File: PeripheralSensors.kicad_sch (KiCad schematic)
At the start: 17 parts, among them J19 TOF_Connectors, J21 IMU_Conn, U2 SAM-M8Q, U4 SP3011-06UTG, U5 SP3011-06UTG, U6 SP3011-06UTG

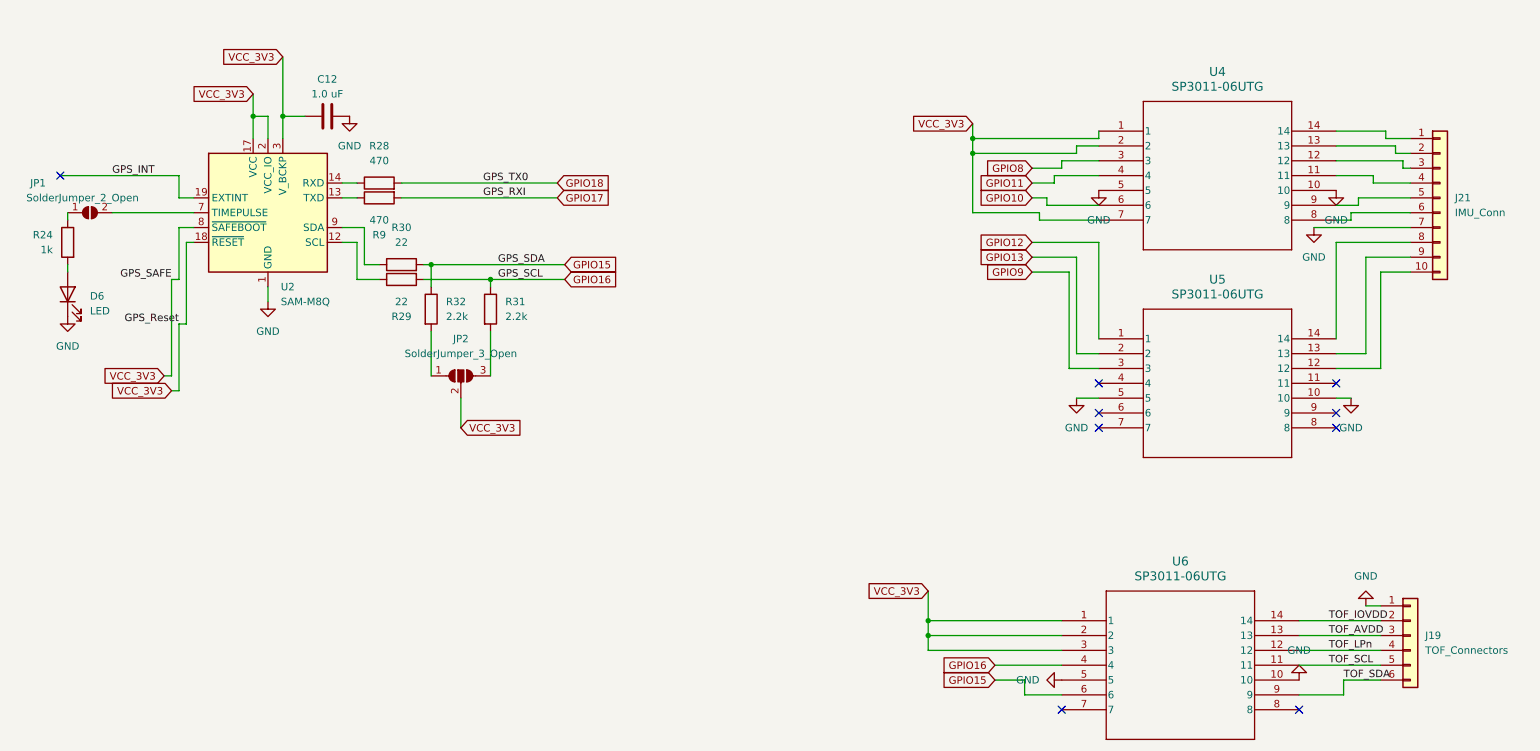
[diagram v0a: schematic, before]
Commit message: pcb draft 2 from billy
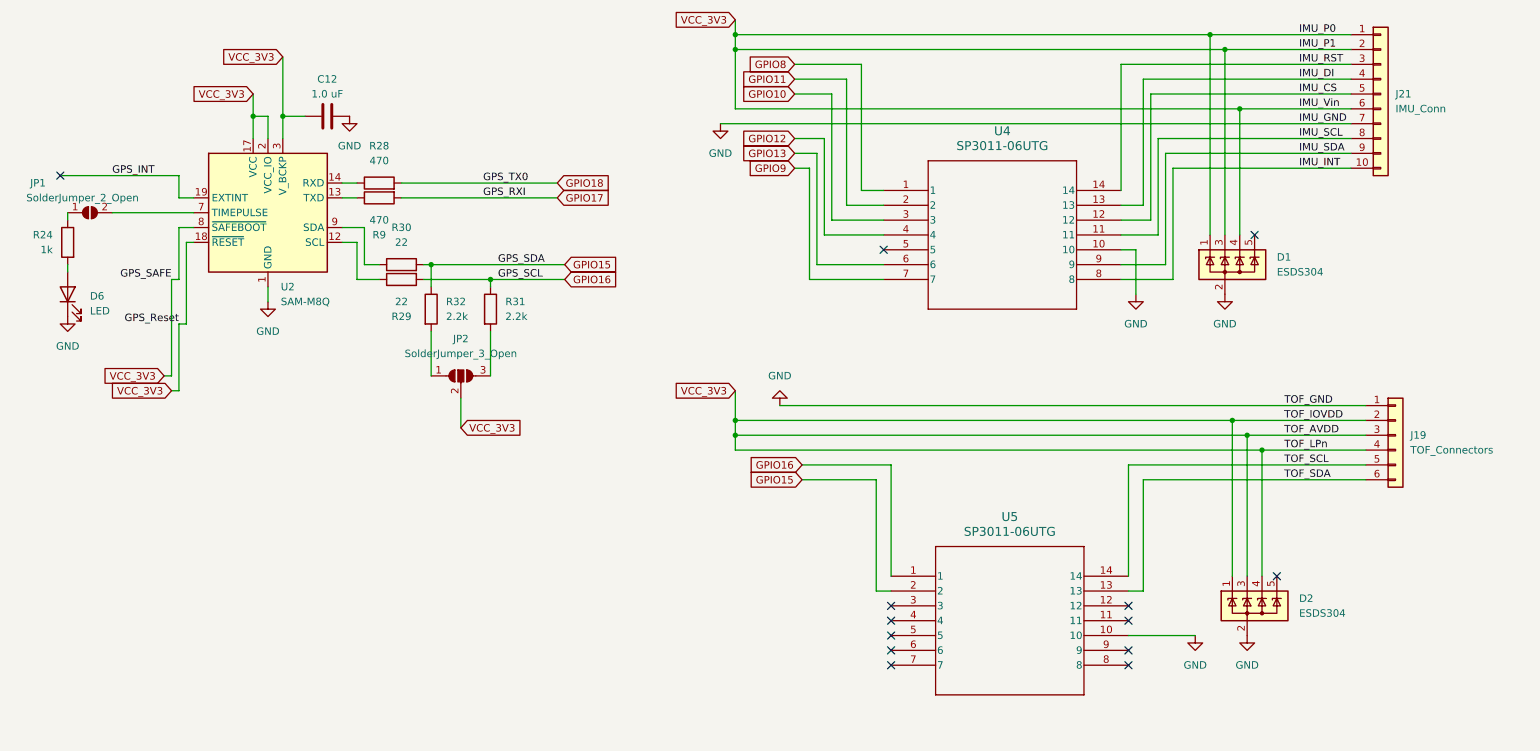
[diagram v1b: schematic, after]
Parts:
- removed U4, U5, U6: SP3011-06UTG, LocalComponents:SON14_SP3011-06UTG_LTF, symbol LocalComps:SP3011-06UTG
- added D1, D2: ESDS304, Package_TO_SOT_SMD:SOT-23-5, symbol Power_Protection:ESDS304
- added U4, U5: SP3011-06UTG, LocalComponents:SON14_SP3011-06UTG_LTF, symbol Custom_Components:SP3011-06UTG
- D6: footprint LocalComponents:LED_LTST-C171_LTO -> LED_SMD:LED_0201_0603Metric
- R24: footprint LocalComponents:RESC1508X55N -> Resistor_SMD:R_0805_2012Metric_Pad1.20x1.40mm_HandSolder
- R28, R9: footprint LocalComponents:RESC6332X65N -> Resistor_SMD:R_0805_2012Metric_Pad1.20x1.40mm_HandSolder
- R29, R30: footprint LocalComponents:R0402 -> Resistor_SMD:R_0805_2012Metric_Pad1.20x1.40mm_HandSolder
- R31, R32: footprint LocalComponents:RESC1005X35N -> Resistor_SMD:R_0805_2012Metric_Pad1.20x1.40mm_HandSolder
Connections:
- net TOF_AVDD is gone; now on net VCC_3V3: J19.3 (Pin_3)
- net TOF_IOVDD is gone; now on net VCC_3V3: J19.2 (Pin_2)
- net TOF_LPn is gone; now on net VCC_3V3: J19.4 (Pin_4)
- net GND: now also D1.2 (A), D2.2 (A), U4.10, U5.10
- net GPIO10: now also U4.3
- net GPIO11: now also U4.2
- net GPIO12: now also U4.4
- net GPIO13: now also U4.6
- net GPIO15: now also U5.2
- net GPIO16: now also U5.1
- net GPIO8: now also U4.1
- net GPIO9: now also U4.7
- net TOF_SCL: now also U5.14
- net TOF_SDA: now also U5.13
- net VCC_3V3: now also J21.1 (Pin_1), J21.2 (Pin_2), J21.6 (Pin_6), D1.1 (K), D1.3 (K), D1.4 (K), D2.1 (K), D2.3 (K), D2.4 (K)
- net IMU_DI: now reaches J21.4 (Pin_4)
- net IMU_DI: now also U4.13
- net IMU_RST: now reaches J21.3 (Pin_3)
- net IMU_RST: now also U4.14
- net IMU_CS: now reaches J21.5 (Pin_5)
- net IMU_CS: now also U4.12
- net IMU_INT: now reaches J21.10 (Pin_10)
- net IMU_INT: now also U4.8
- net IMU_SDA: now reaches J21.9 (Pin_9)
- net IMU_SDA: now also U4.9
- net IMU_SCL: now reaches J21.8 (Pin_8)
- net IMU_SCL: now also U4.11
- no-connect marks 9 -> 13
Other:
- moved on the sheet: J19, J21
